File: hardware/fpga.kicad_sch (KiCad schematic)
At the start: 50 parts, among them J10 Conn_01x03_Pin, J11 Conn_01x03_Pin, J12 Conn_01x10_Pin, J13 Conn_01x02_Pin, J14 Conn_01x03_Pin, J15 Conn_01x02_Pin, J16 Conn_01x03_Pin, U1 ICE40HX4K-TQ144, U2 74HC244

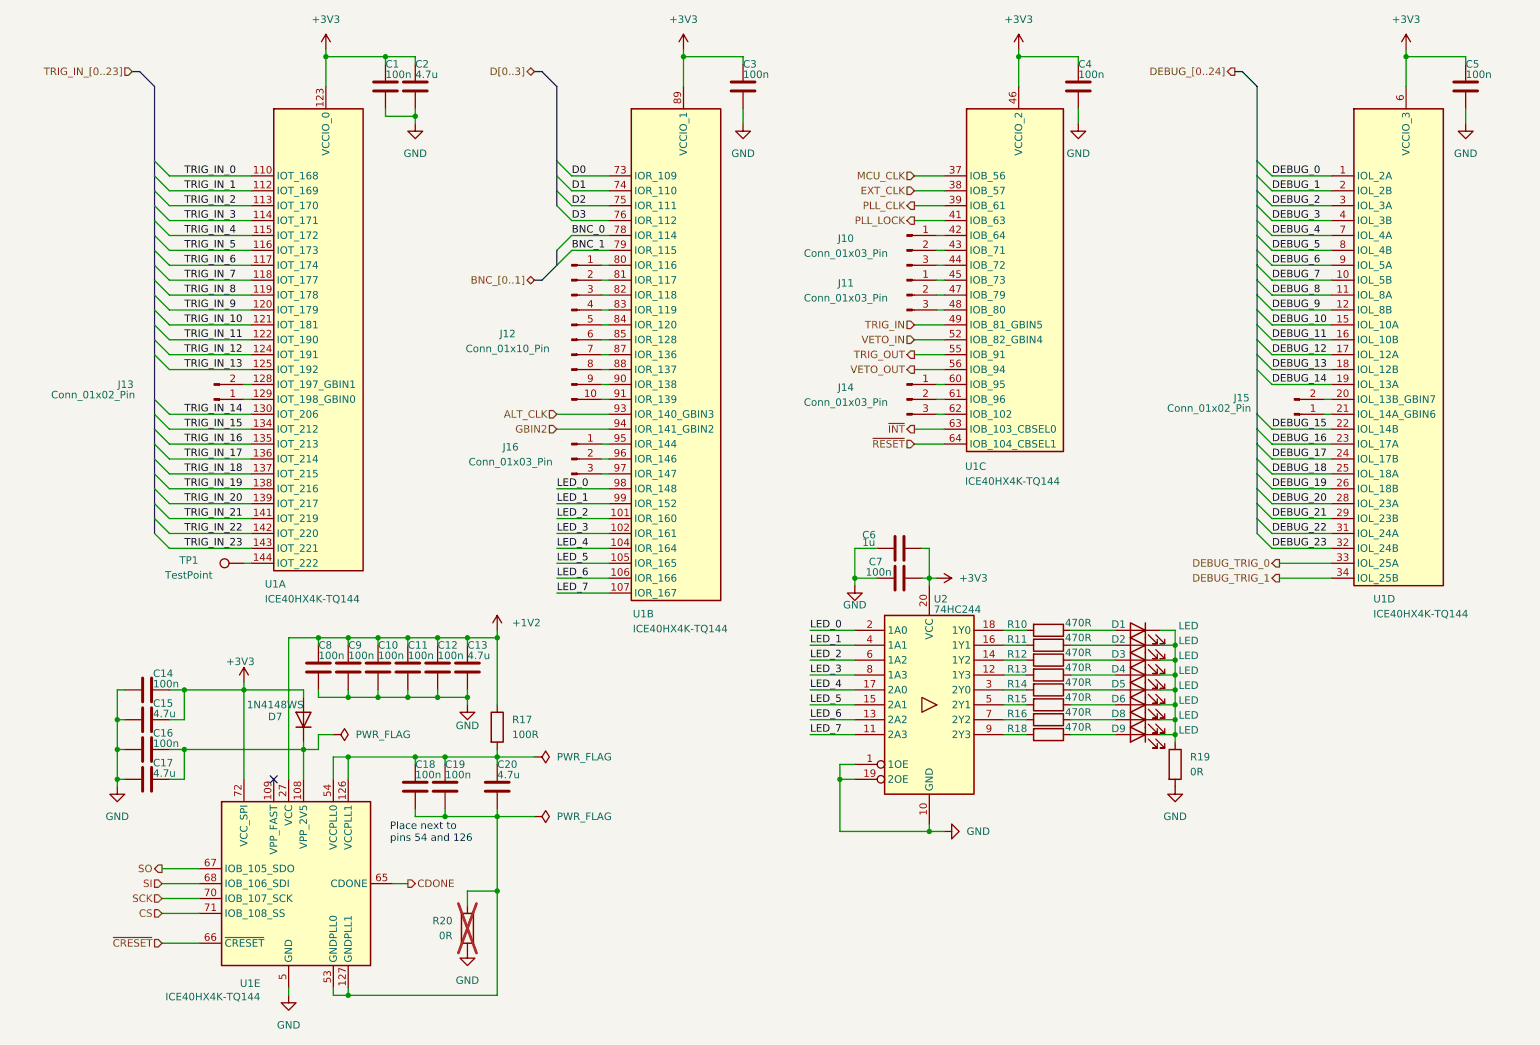
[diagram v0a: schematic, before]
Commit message: route more
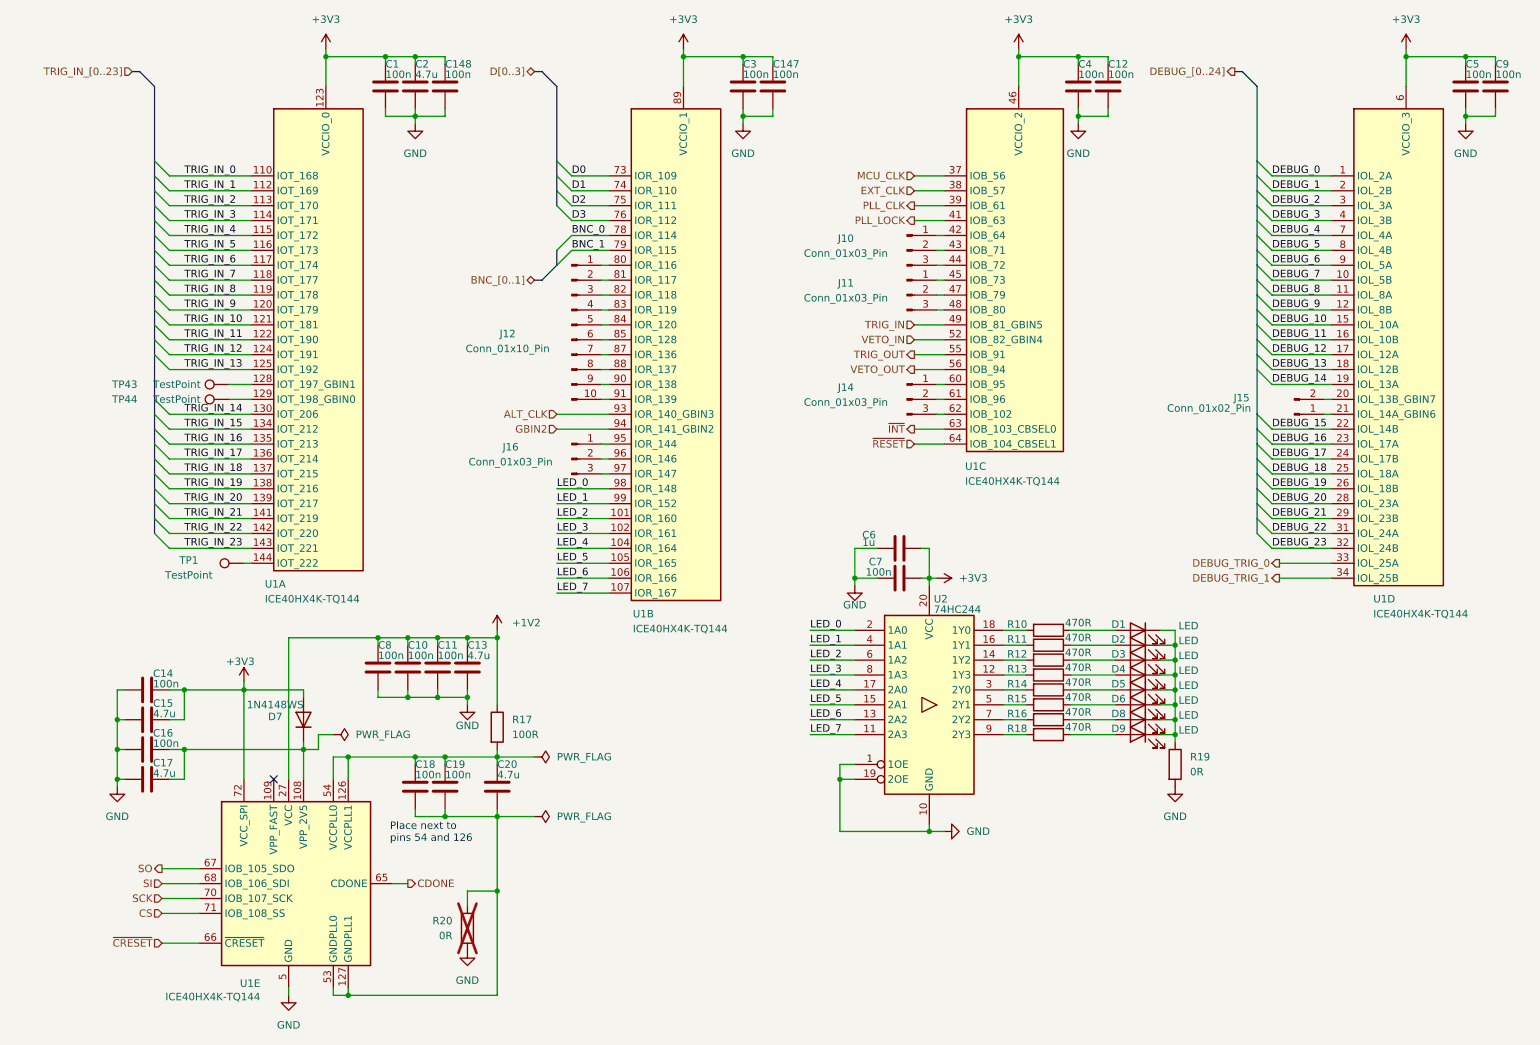
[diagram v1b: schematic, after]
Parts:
- removed J13: Conn_01x02_Pin, Connector_PinHeader_2.54mm:PinHeader_1x02_P2.54mm_Vertical, symbol Connector:Conn_01x02_Pin
- added C147, C148: 100n, Capacitor_SMD:C_0402_1005Metric, symbol Device:C
- added TP43, TP44: TestPoint, TestPoint:TestPoint_Pad_D1.0mm, symbol Connector:TestPoint
- J10, J11, J14, J16: footprint Connector_PinHeader_2.54mm:PinHeader_1x03_P2.54mm_Vertical -> Connector_PinHeader_1.00mm:PinHeader_1x03_P1.00mm_Vertical_SMD_Pin1Left
- J12: footprint Connector_PinHeader_2.54mm:PinHeader_1x10_P2.54mm_Vertical -> Connector_PinHeader_1.00mm:PinHeader_1x10_P1.00mm_Vertical_SMD_Pin1Left
- J15: footprint Connector_PinHeader_2.54mm:PinHeader_1x02_P2.54mm_Vertical -> Connector_PinHeader_1.00mm:PinHeader_1x02_P1.00mm_Vertical_SMD_Pin1Left
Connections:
- net +1V2: no longer C12.1, C9.1
- net +3V3: now also C12.1, C9.1, C147.1, C148.1
- net GND: now also C147.2, C148.2
- net at U1.128 (IOT_197_GBIN1): now also TP43.1
- net at U1.129 (IOT_198_GBIN0): now also TP44.1
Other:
- moved on the sheet: C10, C11, C8
